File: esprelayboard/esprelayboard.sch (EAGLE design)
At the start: 93 parts, among them IC1 MP2315GJ-Z, IC4 CP2104, J1 SM06B-GHS-TB_LF__SN_, J2 SM02B-GHS-TB_LF__SN_, J4 SM06B-GHS-TB_LF__SN_, J6 SM02B-GHS-TB_LF__SN_, J7 SM02B-GHS-TB_LF__SN_, J8 SM02B-GHS-TB_LF__SN_, J9 SM02B-GHS-TB_LF__SN_, K1 G6K-2F-Y, K2 G6K-2F-Y, K4 G6K-2F-Y, Q1 MOSFET-NCHANNELAO3404A, Q2 MOSFET-NCHANNELAO3404A, Q3 MOSFET-NCHANNELAO3404A, Q5 mmbt2222, Q6 mmbt2222, U2 AP2112-3.3, U3 CCS811, X8 ESP32_WROOM32_SKINNY

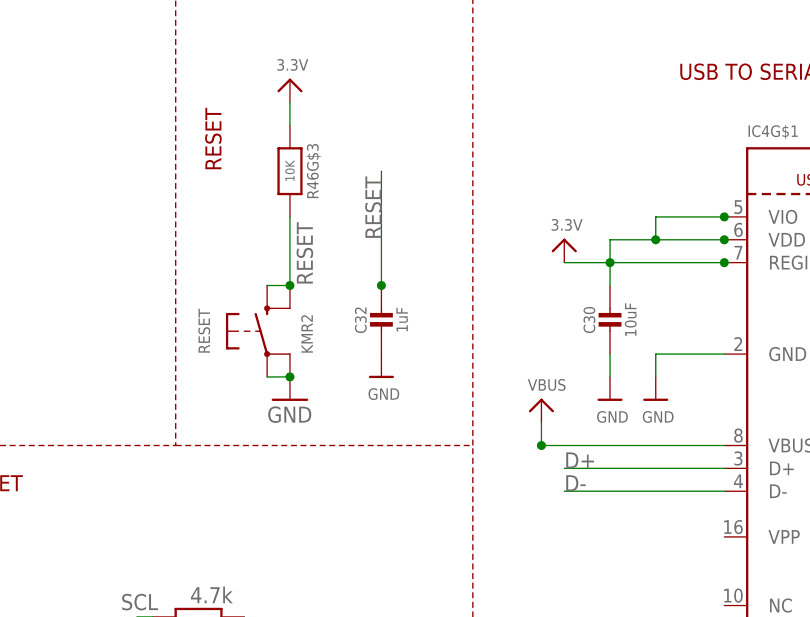
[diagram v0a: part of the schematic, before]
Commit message: final board files
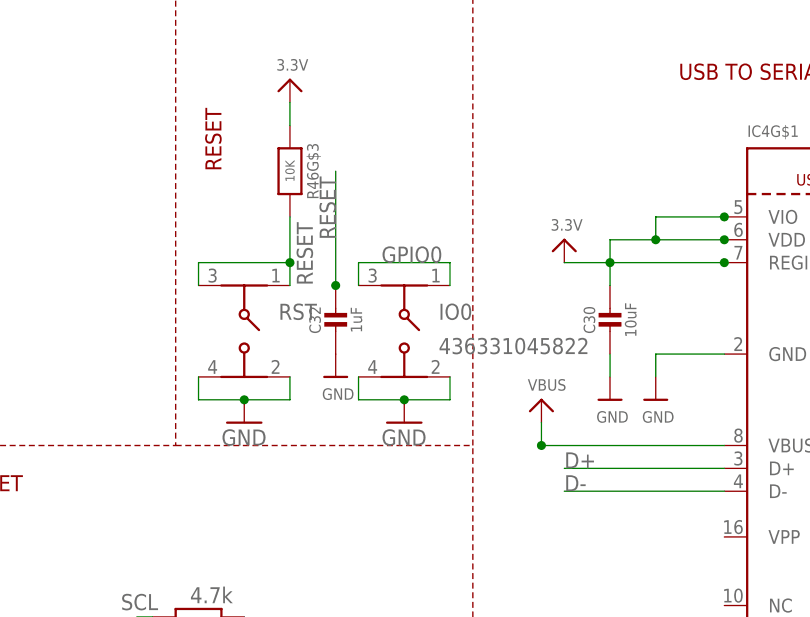
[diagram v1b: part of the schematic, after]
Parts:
- removed RESET: KMR2, microbuilder:SWITCH_TACT_SMT4.6X2.8
- added IO0, RST: 436331045822, 436331045822:436331045822
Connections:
- net GND: now also IO0.2, IO0.4, RST.2, RST.4; no longer RESET.P, RESET.P1
- net GPIO0: now also IO0.1, IO0.3
- net RESET: now also RST.1, RST.3; no longer RESET.S, RESET.S1
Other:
- moved on the sheet: C32
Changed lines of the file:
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@@
 <setting verticaltext="up"/>
 </settings>
-<grid distance="0.01" unitdist="inch" unit="inch" style="lines" multiple="1" display="no" altdistance="0.01" altunitdist="inch" altunit="inch"/>
+<grid distance="0.1" unitdist="inch" unit="inch" style="lines" multiple="1" display="no" altdistance="0.01" altunitdist="inch" altunit="inch"/>
 <layers>
 <layer number="1" name="Top" color="4" fill="1" visible="no" active="no"/>
@@
 <parts>
 <part name="U$14" library="microbuilder" deviceset="3.3V" device=""/>
-<part name="RESET" library="microbuilder" deviceset="SWITCH_TACT_SMT" device="4.6X2.8" value="KMR2"/>
 <part name="GND20" library="supply1" deviceset="GND" device=""/>
 <part name="D13" library="microbuilder" deviceset="LED" device="0805_NOOUTLINE" value="RED"/>
@@
 <part name="C9" library="rcl" library_urn="urn:adsk.eagle:library:334" deviceset="CPOL-US" device="140CLH-1010" package3d_urn="urn:adsk.eagle:package:23391/2"/>
 <part name="U$40" library="microbuilder" deviceset="GND" device=""/>
+<part name="RST" library="436331045822" deviceset="436331045822" device=""/>
+<part name="GND1" library="supply1" deviceset="GND" device=""/>
+<part name="IO0" library="436331045822" deviceset="436331045822" device=""/>
 </parts>
 <sheets>
@@
 <attribute name="VALUE" x="84.836" y="120.396" size="1.27" layer="96"/>
 </instance>
-<instance part="RESET" gate="G$1" x="83.82" y="91.44" smashed="yes" rot="R90">
-<attribute name="NAME" x="77.47" y="88.9" size="1.27" layer="95" rot="R90"/>
-<attribute name="VALUE" x="88.9" y="88.9" size="1.27" layer="96" rot="R90"/>
-</instance>
-<instance part="GND20" gate="1" x="86.36" y="83.82" smashed="yes">
-<attribute name="VALUE" x="83.82" y="81.28" size="1.778" layer="96"/>
+<instance part="GND20" gate="1" x="81.28" y="81.28" smashed="yes">
+<attribute name="VALUE" x="78.74" y="78.74" size="1.778" layer="96"/>
 </instance>
 <instance part="D13" gate="G$1" x="96.52" y="-22.86" smashed="yes" rot="R90">
@@
 <attribute name="VALUE" x="71.12" y="10.16" size="1.016" layer="96" font="vector" ratio="15" align="center"/>
 </instance>
-<instance part="C32" gate="G$1" x="96.52" y="91.44" smashed="yes">
-<attribute name="NAME" x="94.23" y="92.69" size="1.27" layer="95" font="vector" rot="R90" align="center"/>
-<attribute name="VALUE" x="98.82" y="92.69" size="1.27" layer="96" font="vector" rot="R90" align="center"/>
-</instance>
-<instance part="U$52" gate="G$1" x="96.52" y="86.36" smashed="yes">
-<attribute name="VALUE" x="94.996" y="83.82" size="1.27" layer="96"/>
+<instance part="C32" gate="G$1" x="91.44" y="91.44" smashed="yes">
+<attribute name="NAME" x="89.15" y="92.69" size="1.27" layer="95" font="vector" rot="R90" align="center"/>
+<attribute name="VALUE" x="93.74" y="92.69" size="1.27" layer="96" font="vector" rot="R90" align="center"/>
+</instance>
+<instance part="U$52" gate="G$1" x="91.44" y="86.36" smashed="yes">
+<attribute name="VALUE" x="89.916" y="83.82" size="1.27" layer="96"/>
 </instance>
 <instance part="IC4" gate="G$1" x="149.86" y="83.82" smashed="yes">
@@
 <instance part="U$40" gate="G$1" x="-36.068" y="2.794" smashed="yes">
 <attribute name="VALUE" x="-37.592" y="0.254" size="1.27" layer="96"/>
+</instance>
+<instance part="RST" gate="G$1" x="81.28" y="91.44" smashed="yes">
+<attribute name="NAME" x="85.09" y="92.71" size="1.778" layer="95"/>
+</instance>
+<instance part="GND1" gate="1" x="99.06" y="81.28" smashed="yes">
+<attribute name="VALUE" x="96.52" y="78.74" size="1.778" layer="96"/>
+</instance>
+<instance part="IO0" gate="G$1" x="99.06" y="91.44" smashed="yes">
+<attribute name="NAME" x="102.87" y="92.71" size="1.778" layer="95"/>
+<attribute name="VALUE" x="102.87" y="88.9" size="1.778" layer="96"/>
 </instance>
 </instances>
@@
 <nets>
 <net name="GND" class="0">
-<segment>
-<pinref part="RESET" gate="G$1" pin="P"/>
-<pinref part="RESET" gate="G$1" pin="P1"/>
-<wire x1="83.82" y1="86.36" x2="86.36" y2="86.36" width="0.1524" layer="91"/>
-<pinref part="GND20" gate="1" pin="GND"/>
-<junction x="86.36" y="86.36"/>
-</segment>
 <segment>
 <pinref part="U$45" gate="G$1" pin="GND"/>
@@
 <pinref part="C9" gate="G$1" pin="-"/>
 <pinref part="U$40" gate="G$1" pin="GND"/>
+</segment>
+<segment>
+<pinref part="RST" gate="G$1" pin="2"/>
+<wire x1="76.2" y1="86.36" x2="76.2" y2="83.82" width="0.1524" layer="91"/>
+<pinref part="GND20" gate="1" pin="GND"/>
+<wire x1="76.2" y1="83.82" x2="81.28" y2="83.82" width="0.1524" layer="91"/>
+<pinref part="RST" gate="G$1" pin="4"/>
+<wire x1="81.28" y1="83.82" x2="86.36" y2="83.82" width="0.1524" layer="91"/>
+<wire x1="86.36" y1="83.82" x2="86.36" y2="86.36" width="0.1524" layer="91"/>
+<junction x="81.28" y="83.82"/>
+</segment>
+<segment>
+<pinref part="GND1" gate="1" pin="GND"/>
+<pinref part="IO0" gate="G$1" pin="2"/>
+<wire x1="93.98" y1="86.36" x2="93.98" y2="83.82" width="0.1524" layer="91"/>
+<wire x1="93.98" y1="83.82" x2="99.06" y2="83.82" width="0.1524" layer="91"/>
+<pinref part="IO0" gate="G$1" pin="4"/>
+<wire x1="104.14" y1="86.36" x2="104.14" y2="83.82" width="0.1524" layer="91"/>
+<wire x1="104.14" y1="83.82" x2="99.06" y2="83.82" width="0.1524" layer="91"/>
+<junction x="99.06" y="83.82"/>
 </segment>
 </net>
@@
 <net name="RESET" class="0">
 <segment>
-<wire x1="86.36" y1="104.14" x2="86.36" y2="96.52" width="0.1524" layer="91"/>
+<wire x1="86.36" y1="104.14" x2="86.36" y2="99.06" width="0.1524" layer="91"/>
 <label x="88.9" y="96.52" size="1.778" layer="95" rot="R90"/>
-<pinref part="RESET" gate="G$1" pin="S1"/>
-<pinref part="RESET" gate="G$1" pin="S"/>
-<wire x1="86.36" y1="96.52" x2="83.82" y2="96.52" width="0.1524" layer="91"/>
-<junction x="86.36" y="96.52"/>
 <pinref part="R46" gate="G$3" pin="2"/>
+<pinref part="RST" gate="G$1" pin="3"/>
+<pinref part="RST" gate="G$1" pin="1"/>
+<wire x1="86.36" y1="99.06" x2="86.36" y2="96.52" width="0.1524" layer="91"/>
+<wire x1="76.2" y1="96.52" x2="76.2" y2="99.06" width="0.1524" layer="91"/>
+<wire x1="76.2" y1="99.06" x2="86.36" y2="99.06" width="0.1524" layer="91"/>
+<junction x="86.36" y="99.06"/>
 </segment>
 <segment>
@@
 <segment>
 <pinref part="C32" gate="G$1" pin="1"/>
-<wire x1="96.52" y1="96.52" x2="96.52" y2="109.22" width="0.1524" layer="91"/>
-<label x="96.52" y="101.6" size="1.778" layer="95" rot="R90"/>
-<junction x="96.52" y="96.52"/>
+<wire x1="91.44" y1="96.52" x2="91.44" y2="109.22" width="0.1524" layer="91"/>
+<label x="91.44" y="101.6" size="1.778" layer="95" rot="R90"/>
+<junction x="91.44" y="96.52"/>
 </segment>
 </net>
@@
 <pinref part="X8" gate="G$1" pin="IO0/A2_1"/>
 </segment>
+<segment>
+<pinref part="IO0" gate="G$1" pin="1"/>
+<wire x1="93.98" y1="96.52" x2="93.98" y2="99.06" width="0.1524" layer="91"/>
+<pinref part="IO0" gate="G$1" pin="3"/>
+<wire x1="104.14" y1="96.52" x2="104.14" y2="99.06" width="0.1524" layer="91"/>
+<wire x1="104.14" y1="99.06" x2="93.98" y2="99.06" width="0.1524" layer="91"/>
+<label x="96.52" y="99.06" size="1.778" layer="95"/>
+</segment>
 </net>
